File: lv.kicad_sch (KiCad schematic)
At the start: 8 parts, among them J5 CAN_NANO_01x05, J6 CAN_NANO_01x05, J7 CarLVPowerConnector, J8 CAN_DEBUG_NANO_01x04

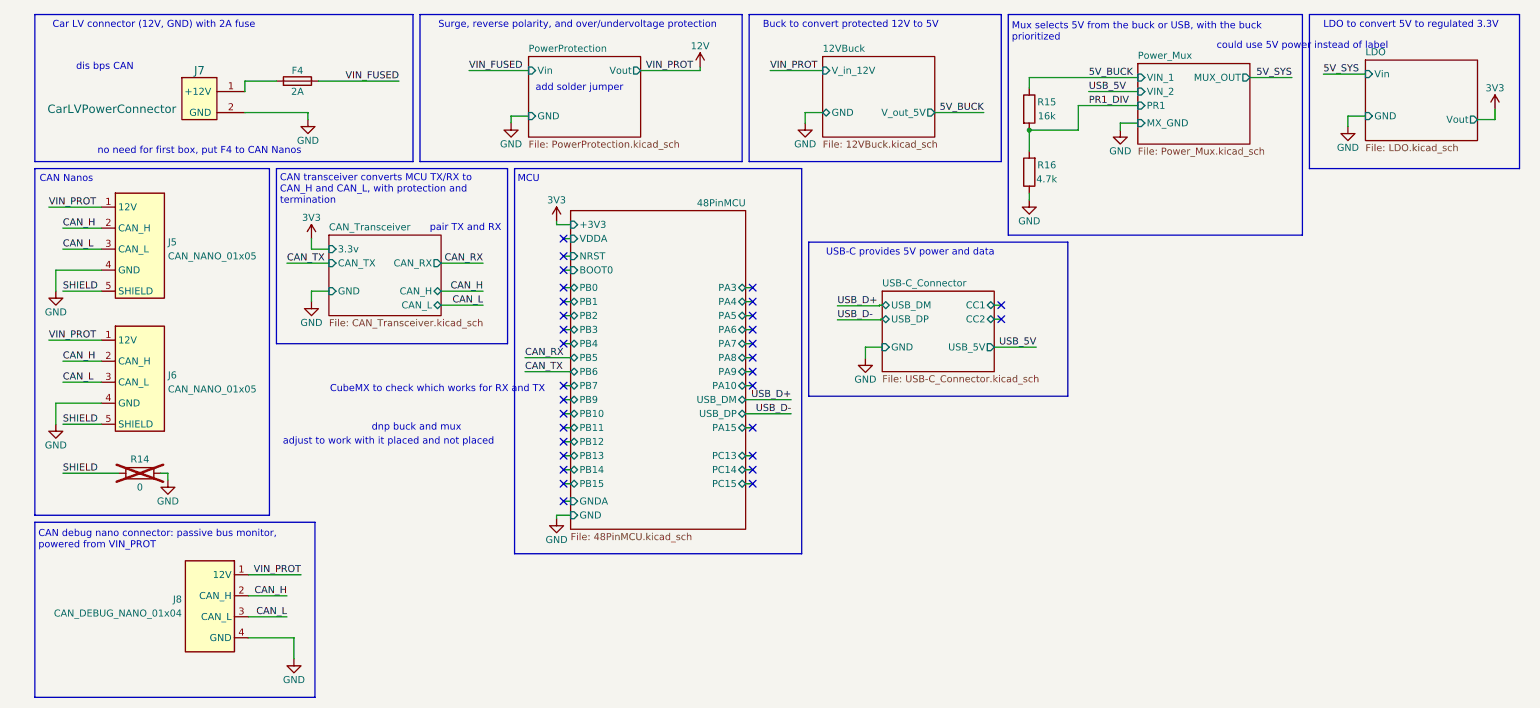
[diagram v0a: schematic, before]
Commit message: fixed lv
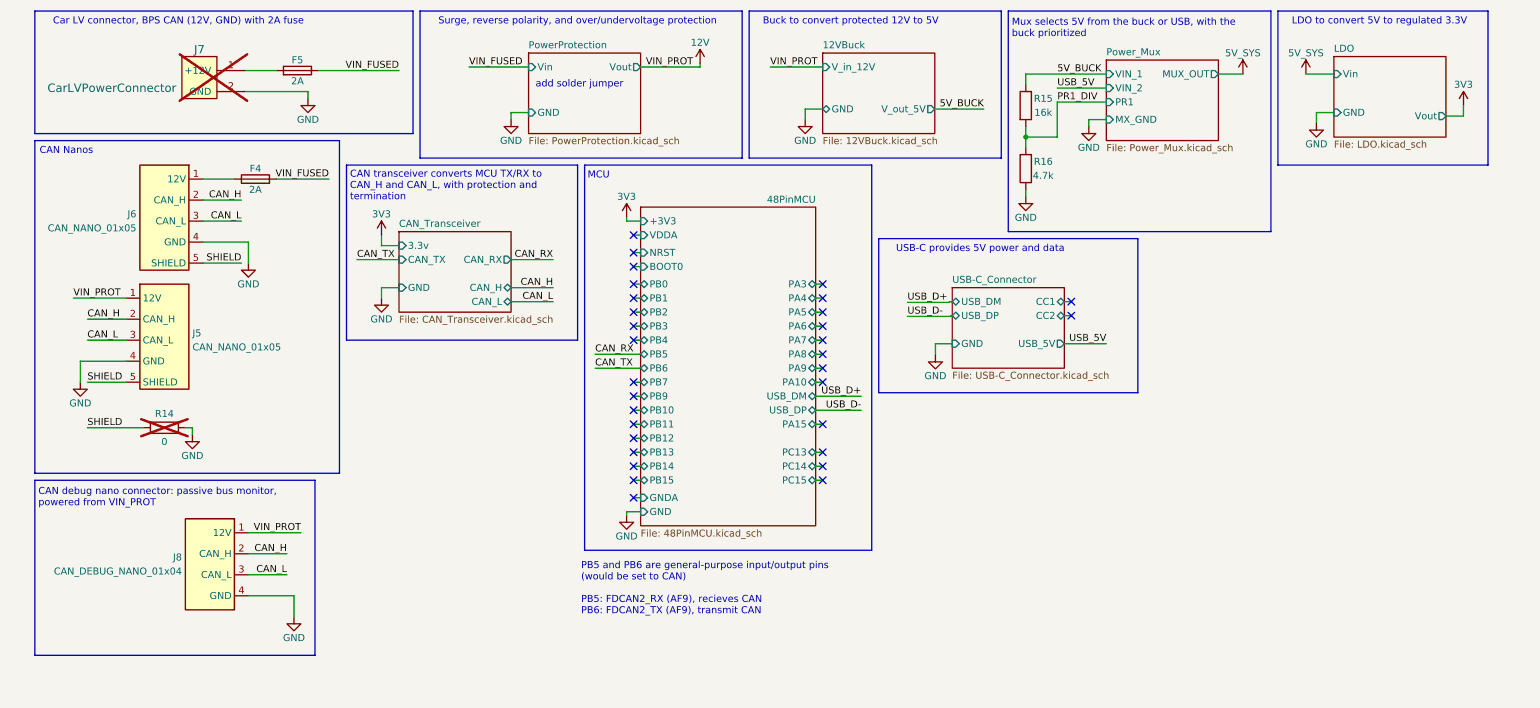
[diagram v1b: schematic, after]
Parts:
- added F5: 2A, LHRS_Power:Fuse-3557-2, symbol lhrs_power:Fuse_3557_2
- J7: now not fitted
- renumbered J6 to J5, J5 to J6
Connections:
- net 12V: no longer J6.1 (12V)
- net VIN_FUSED: now also F4.1, F5.2; no longer F4.2
- net at J7.1 (+12V): now also F5.1; no longer F4.1
- new net: F4.2, J6.1 (12V)
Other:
- note added: "Car LV connector, BPS CAN (12V, GND) with 2A fuse"
- note added: "PB5 and PB6 are general-purpose input/output pins (would be set to CAN) PB5: FDCAN2_RX (AF9), recieves CAN PB6: FDCAN2_TX (AF9), transmit CAN"
- note removed: "Car LV connector (12V, GND) with 2A fuse"
- note removed: "CubeMX to check which works for RX and TX"
- note removed: "adjust to work with it placed and not placed"
- note removed: "could use 5V power instead of label"
- note removed: "dis bps CAN"
- note removed: "dnp buck and mux"
- note removed: "no need for first box, put F4 to CAN Nanos"
- note removed: "pair TX and RX"
- moved on the sheet: J5, J6, J8, R14, R15, R16

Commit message: shifted hierarchical sheets
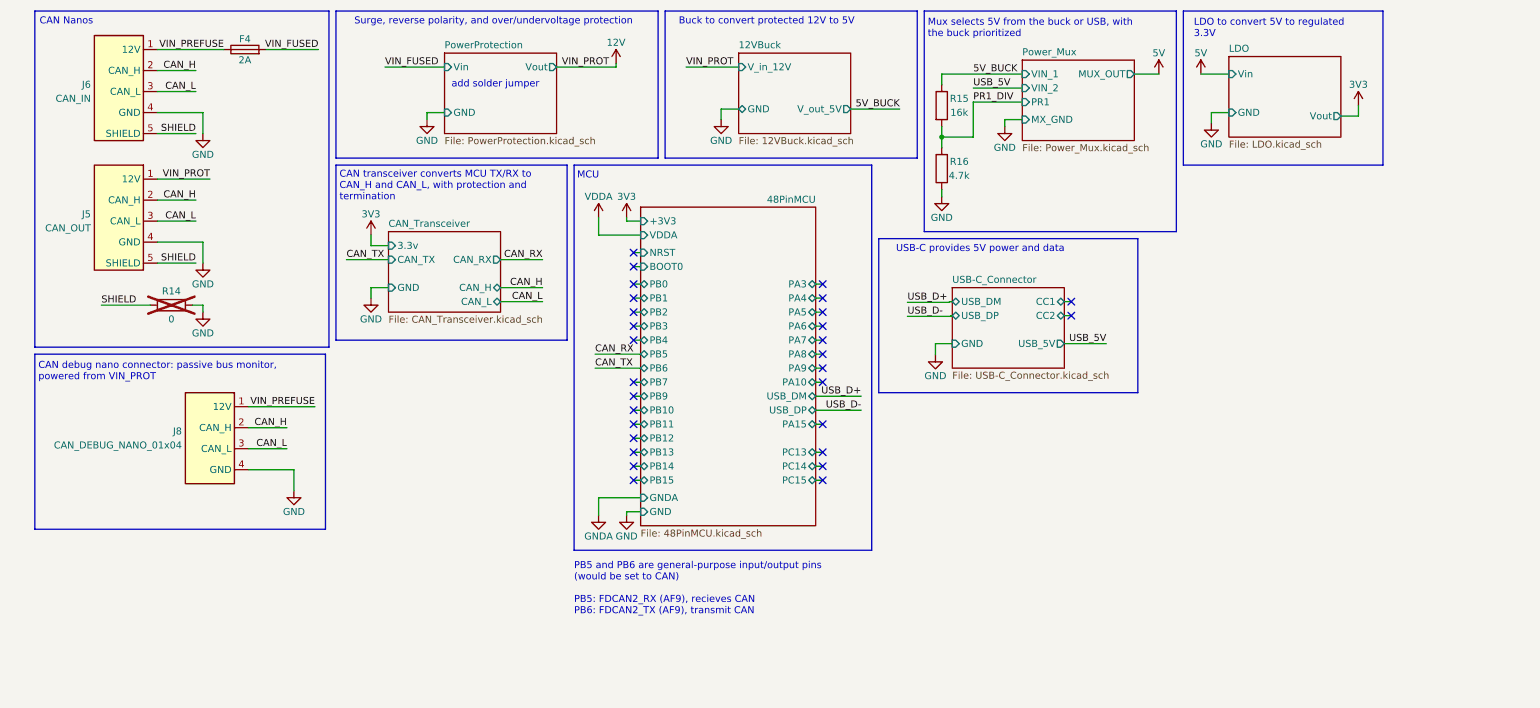
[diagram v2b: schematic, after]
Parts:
- removed F5: 2A, LHRS_Power:Fuse-3557-2, symbol lhrs_power:Fuse_3557_2
- removed J7: CarLVPowerConnector, LHRS_Connectors:Molex_Nano-Fit_105309-xx02_1x02_P2.50mm_Vertical, symbol lhrs_connectors:CarLVPowerConnector
- J5: value CAN_NANO_01x05 -> CAN_OUT
- J6: value CAN_NANO_01x05 -> CAN_IN
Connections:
- net 12V: no longer J8.1 (12V)
- net VIN_PREFUSE: now reaches F4.2, J6.1 (12V)
- net VIN_PREFUSE: now also J8.1 (12V)
- no-connect marks 31 -> 29
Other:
- note removed: "Car LV connector, BPS CAN (12V, GND) with 2A fuse"
- moved on the sheet: F4, J5, J6, J8, R14, R15, R16
